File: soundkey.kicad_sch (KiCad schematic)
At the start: 23 parts, among them J1 Conn_01x01_Socket, J2 Conn_01x06_Socket, J3 Conn_01x01_Socket, Q1 AO3401A, U1 XC6206PxxxMR, U2 TP4057, U3 MSM381ACB026, U4 CHR11

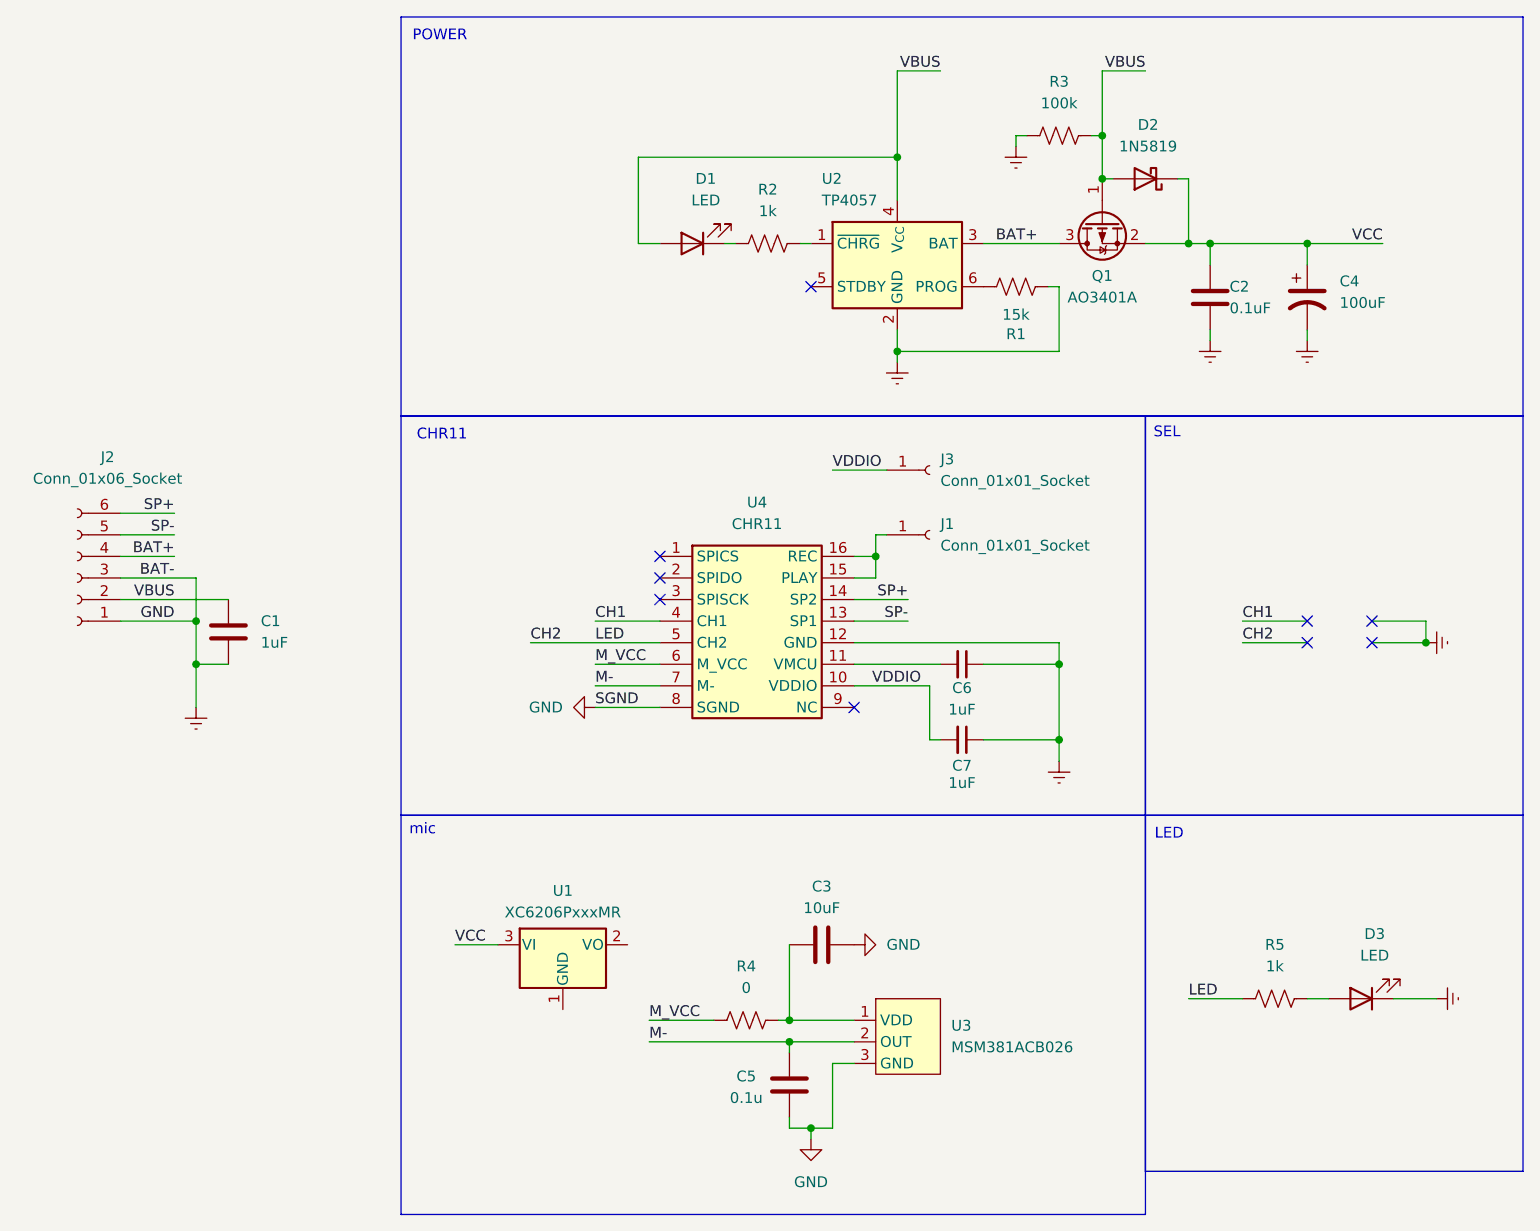
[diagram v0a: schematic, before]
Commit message: 2608261612_chg arch.
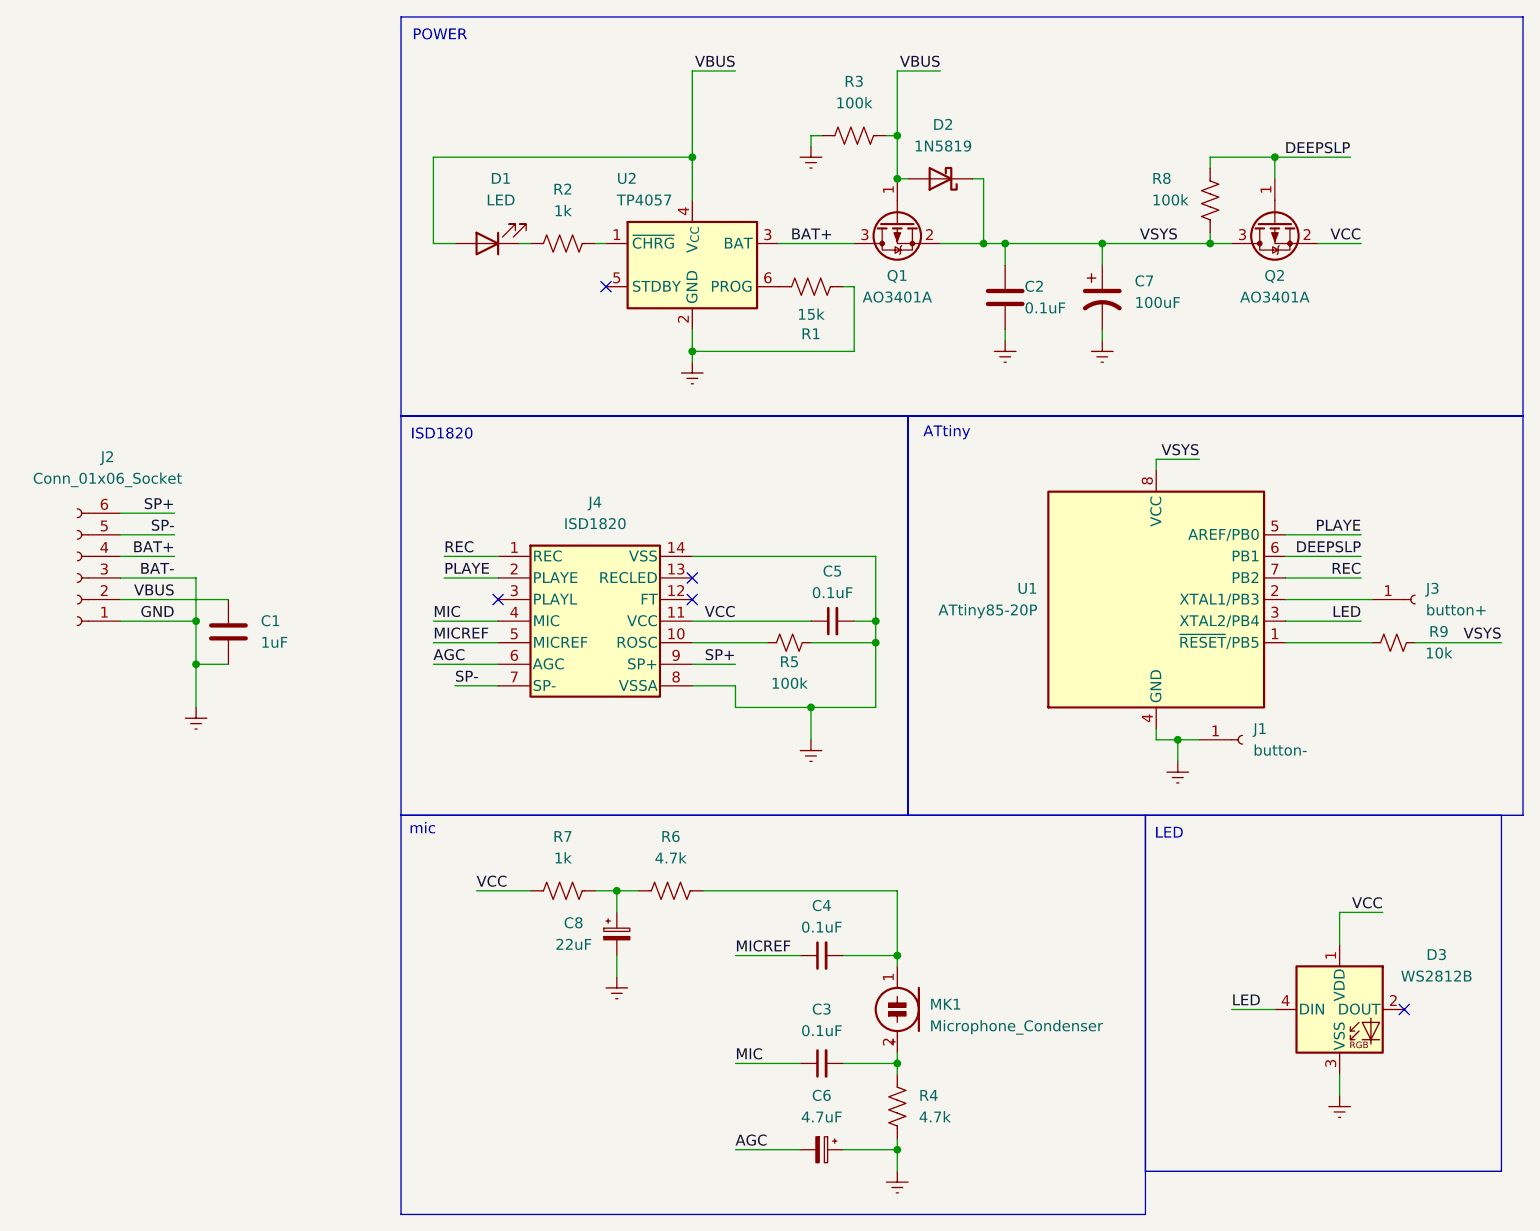
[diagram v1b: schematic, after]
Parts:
- removed C3: 10uF, symbol Device:C
- removed C5: 0.1u, symbol Device:C
- removed C6, C7: 1uF, symbol Device:C_Small
- removed D3: LED, symbol Device:LED
- removed R5: 1k, symbol Device:R_US
- removed U1: XC6206PxxxMR, Package_TO_SOT_SMD:SOT-23-3, symbol Regulator_Linear:XC6206PxxxMR
- removed U3: MSM381ACB026, symbol 1_New_Library_0:MSM381ACB026
- removed U4: CHR11, Package_SO:SOIC-16_3.9x9.9mm_P1.27mm, symbol 1_New_Library_0:CHR11
- added C3, C4, C5: 0.1uF, symbol Device:C_Small
- added C6: 4.7uF, symbol Device:C_Polarized_Small
- added C8: 22uF, symbol Device:C_Polarized_Small
- added D3: WS2812B, LED_SMD:LED_WS2812B_PLCC4_5.0x5.0mm_P3.2mm, symbol LED:WS2812B
- added J4: ISD1820, Package_DIP:DIP-14_W7.62mm_Socket, symbol 1_New_Library_0:ISD1820
- added MK1: Microphone_Condenser, symbol Device:Microphone_Condenser
- added Q2: AO3401A, Package_TO_SOT_SMD:SOT-23, symbol Transistor_FET:AO3401A
- added R5: 100k, symbol Device:R_Small_US
- added R6: 4.7k, symbol Device:R_US
- added R7: 1k, symbol Device:R_US
- added R8: 100k, symbol Device:R_US
- added R9: 10k, symbol Device:R_Small_US
- added U1: ATtiny85-20P, Package_DIP:DIP-8_W7.62mm, symbol MCU_Microchip_ATtiny:ATtiny85-20P
- J1: value Conn_01x01_Socket -> button-
- J3: value Conn_01x01_Socket -> button+
- R4: value 0 -> 4.7k
- renumbered C4 to C7
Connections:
- net M_VCC is gone; now on net Earth: R4.1
- net Earth: now also J1.1 (Pin_1), C5.2, C6.1, C8.2, D3.3 (VSS), J4.14 (VSS), J4.8 (VSSA), R5.2, U1.4 (GND)
- net SP+: now also J4.9 (SP+)
- net SP-: now also J4.7 (SP-)
- net VCC: now also C5.1, D3.1 (VDD), J4.11 (VCC), Q2.2 (S), R7.2; no longer C2.1, C7.1, D2.1 (K), Q1.2 (S)
- net at R4.2: now also C3.2, MK1.2 (+)
- net VDDIO: no longer names the net of J3.1 (Pin_1)
- net VDDIO: now also U1.2 (XTAL1/PB3)
- new net: R9.1, U1.1 (~{RESET}/PB5)
- new net: C4.2, MK1.1 (-), R6.1
- new net: C8.1, R6.2, R7.1
- new net: J4.10 (ROSC), R5.1
- new net AGC: C6.2, J4.6 (AGC)
- new net DEEPSLP: Q2.1 (G), R8.2, U1.6 (PB1)
- new net LED: D3.4 (DIN), U1.3 (XTAL2/PB4)
- new net MIC: C3.1, J4.4 (MIC)
- new net MICREF: C4.1, J4.5 (MICREF)
- new net PLAYE: J4.2 (PLAYE), U1.5 (AREF/PB0)
- new net REC: J4.1 (REC), U1.7 (PB2)
- new net VSYS: C2.1, C7.1, D2.1 (K), Q1.2 (S), Q2.3 (D), R8.1, R9.2, U1.8 (VCC)
- no-connect marks 9 -> 5
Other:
- note added: "ATtiny"
- note added: "ISD1820"
- note removed: "CHR11"
- note removed: "SEL"
- moved on the sheet: C2, C7, D1, D2, Q1, R1, R2, R3, U2
